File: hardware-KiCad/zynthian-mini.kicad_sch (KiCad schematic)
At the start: 37 parts, among them SW1 SW_Push, SW2 SW_Push, SW3 SW_Push, SW4 SW_Push, U1 74HCT14, U2 H11L1M

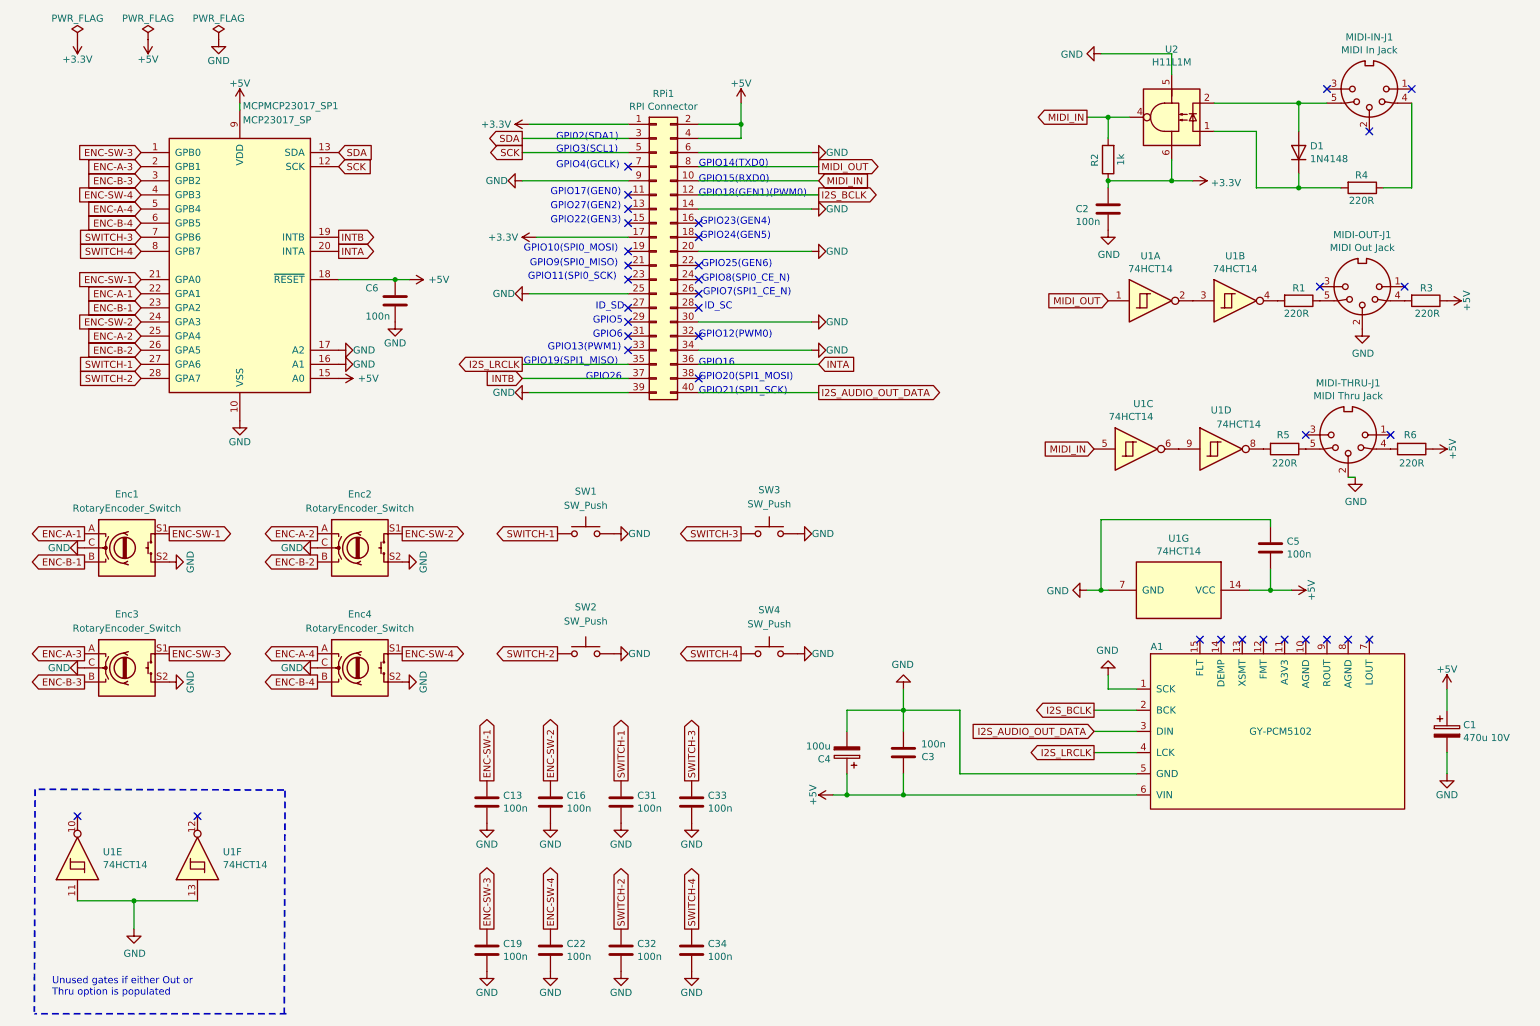
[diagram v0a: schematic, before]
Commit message: reverted back to v1-beta version for saving it into its own branch
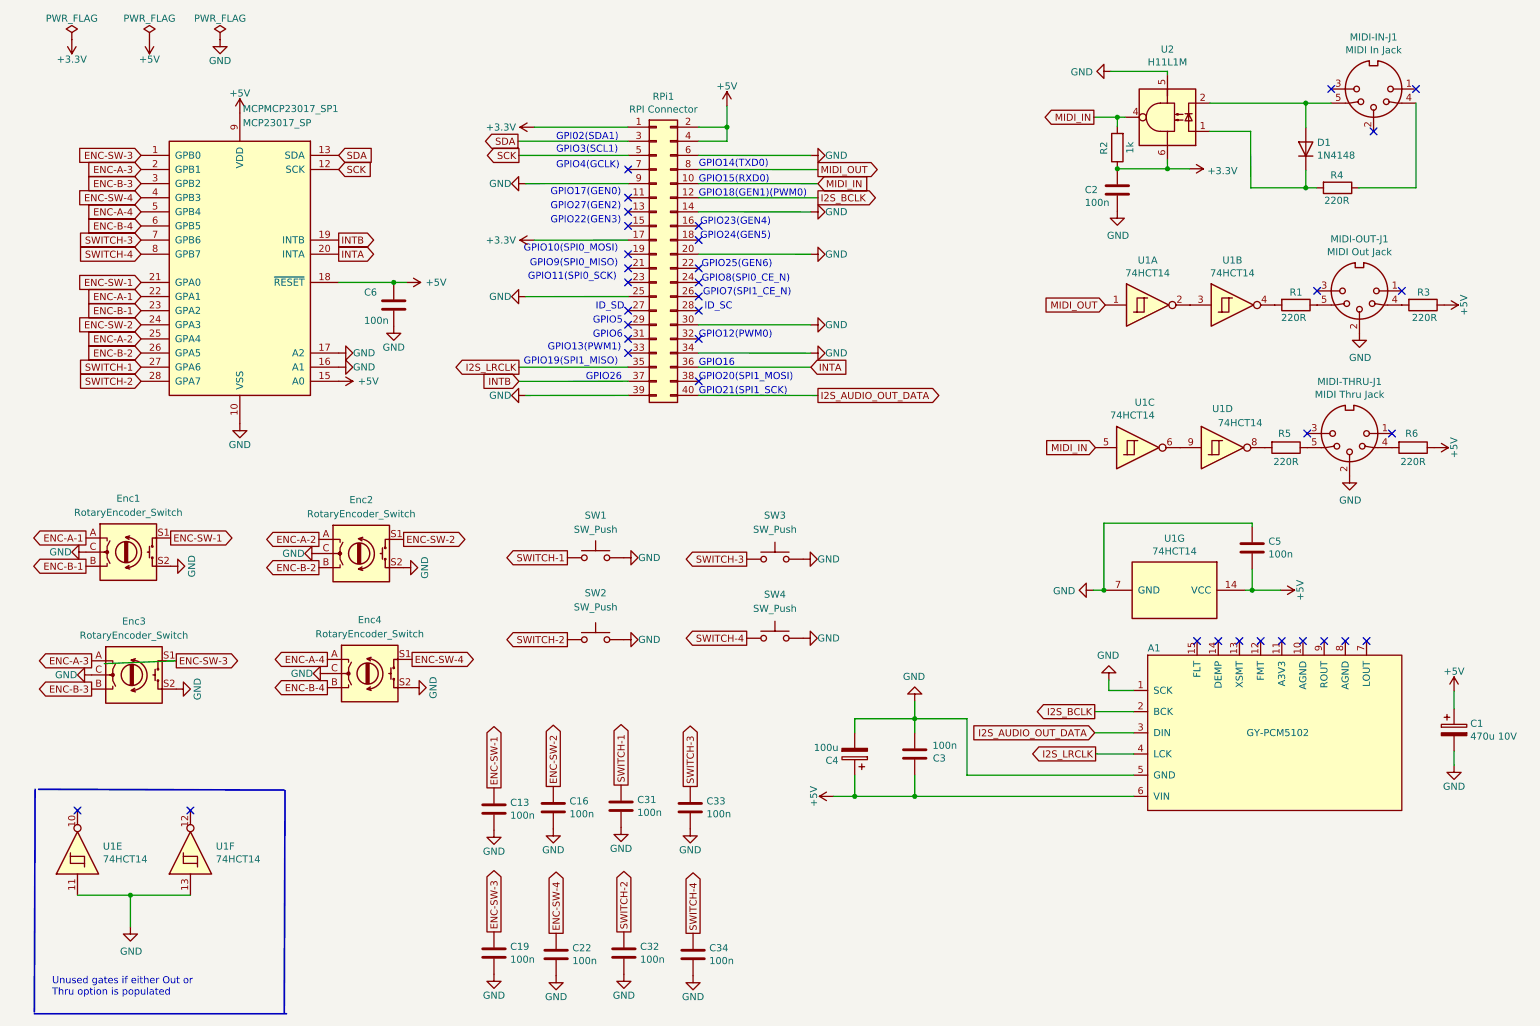
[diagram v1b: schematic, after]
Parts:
- A1: footprint project-footprints:GY-PCM5102 -> clumsyMIDI:GY-PCM5102
- MIDI-IN-J1, MIDI-OUT-J1, MIDI-THRU-J1: footprint project-footprints:MultiDIN5 -> My-Library:MultiDIN5
- SW1, SW2, SW3, SW4: footprint project-footprints:push-button -> My-Library:push-button
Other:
- moved on the sheet: A1, C1, C13, C16, C19, C2, C22, C3, C31, C32, C33, C34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
